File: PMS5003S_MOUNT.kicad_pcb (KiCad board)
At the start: 2 copper layers, 90 x 90 mm, 14 parts, among them J1 CONN_MCU, J2 CONN_PMS, U1 USB_PCB

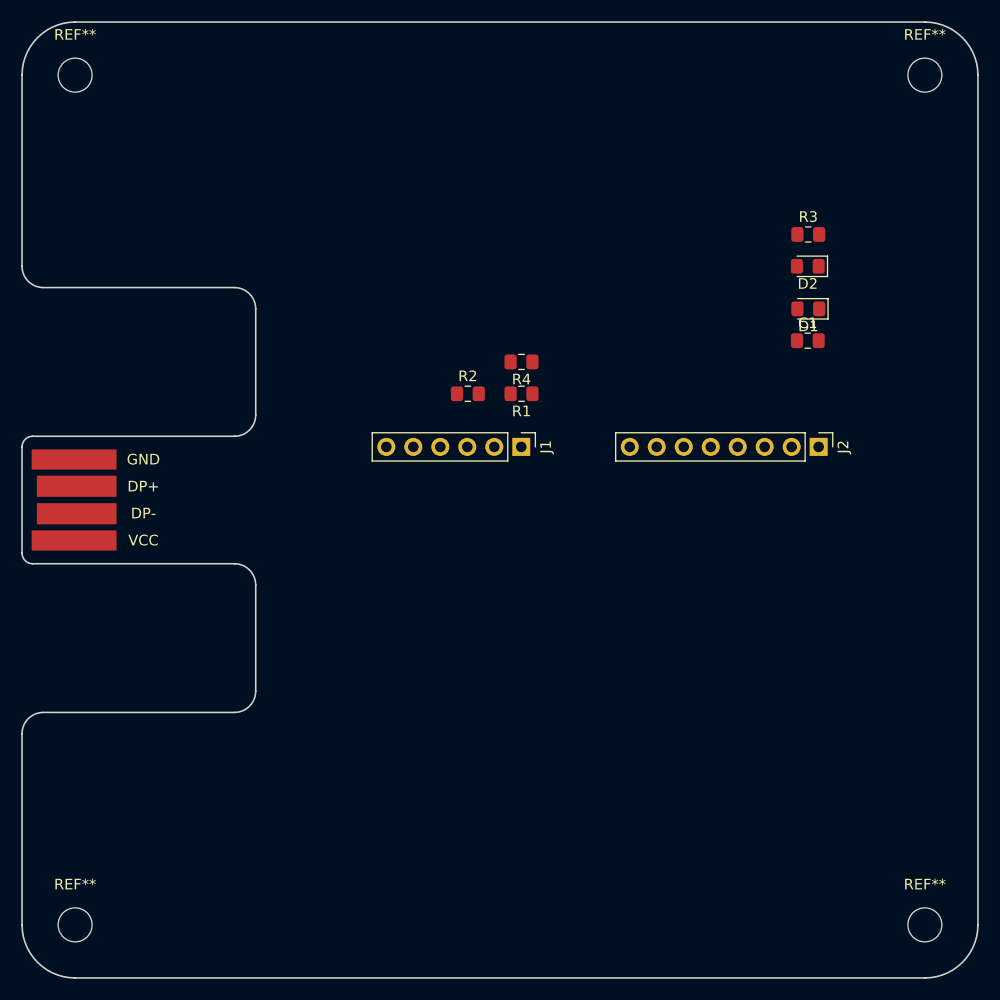
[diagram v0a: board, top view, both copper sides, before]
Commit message: update,
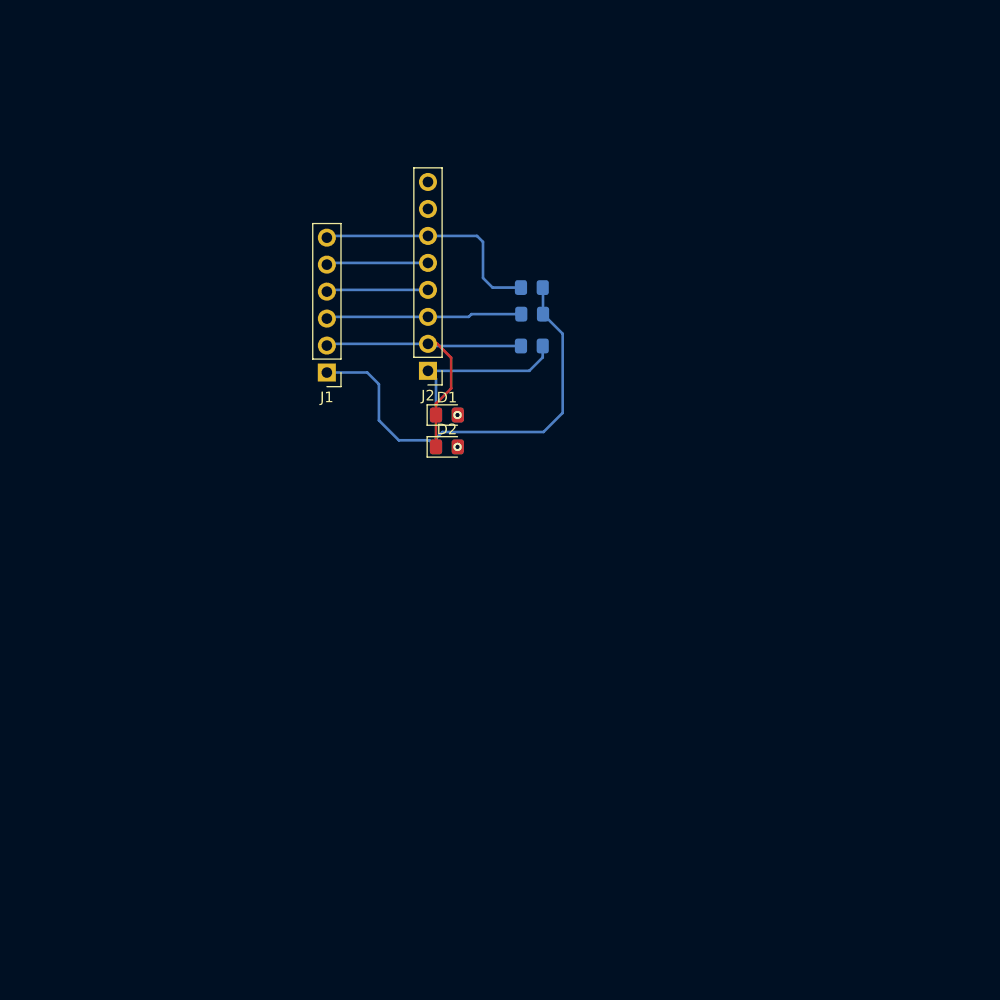
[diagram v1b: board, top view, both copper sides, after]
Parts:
- removed REF** (x4): MountingHole_3.2mm_M3_DIN965, MountingHole:MountingHole_3.2mm_M3_DIN965
- removed U1: USB_PCB, footprint-lib.pretty:usb-PCB
- C1, R1, R2, R3, R4: moved to B.Cu
- J2: footprint Connector_PinHeader_2.54mm:PinHeader_1x08_P2.54mm_Vertical -> footprint-lib:PMS5003S
- moved R3 38.0 mm to (45.0, 42.0)
- moved D2 38.0 mm to (45.0, 45.0), turned to 0 degrees
- moved D1 35.5 mm to (45.0, 42.0), turned to 0 degrees
- moved C1 26.0 mm to (53.0, 35.5), turned to 180 degrees
- moved J1 19.6 mm to (33.7, 38.0), turned to 180 degrees
- moved R2 11.7 mm to (53.0, 30.0)
- moved R4 10.6 mm to (45.0, 45.0), turned to 0 degrees
- moved J2 8.77 mm to (74.0, 38.6), turned to 90 degrees
- moved R1 7.57 mm to (53.0, 32.5)
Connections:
- J2 pad 7: Net-(J2-Pad7) -> (no net)
- J2 pad 8: Net-(J2-Pad8) -> (no net)
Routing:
- net +3V3: track 0.00 -> 41.5 mm
- net GND: track 0.00 -> 30.1 mm
- net /SEN_RESET: track 0.00 -> 22.6 mm
- net /SEN_SET: track 0.00 -> 18.5 mm
- net +5V: track 0.00 -> 16.9 mm
- net /SEN_TXD: track 0.00 -> 9.59 mm
- net /SEN_RXD: track 0.00 -> 9.59 mm
- net Net-(D2-Pad2): vias 0 -> 1
- net Net-(D1-Pad2): vias 0 -> 1
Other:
- board outline removed
- board text removed: "PMS5003S"
